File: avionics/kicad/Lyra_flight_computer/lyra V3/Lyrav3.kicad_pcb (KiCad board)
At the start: 4 copper layers, 50 x 60 mm, 110 parts, among them J1 Conn_01x10, J10 TSW-104-08-T-T-RA, J11 Screw_Terminal_01x12, J12 Screw_Terminal_01x12, J13 Conn_01x10, J2 Conn_01x02, J3 Conn_01x07, J4 Conn_01x03, J5 Conn_01x05, J6 USB_B_Micro, J8 Conn_01x05, J9 Conn_01x02, Q1 AO3401A, Q2 KY6802, Q3 KY6802, U1 AMS1117-5.0, U10 ADS1015IDGS, U11 PCF8574, U2 AMS1117-3.3, U3 W25Q64JVXGIQ, U4 BMI088, U5 MPL3115A2, U6 ADXL375BCCZ-RL7, U7 LIS3MDL, U8 RP2040, U9 ADS1015IDGS, X1 S3D12.288000B20F30T

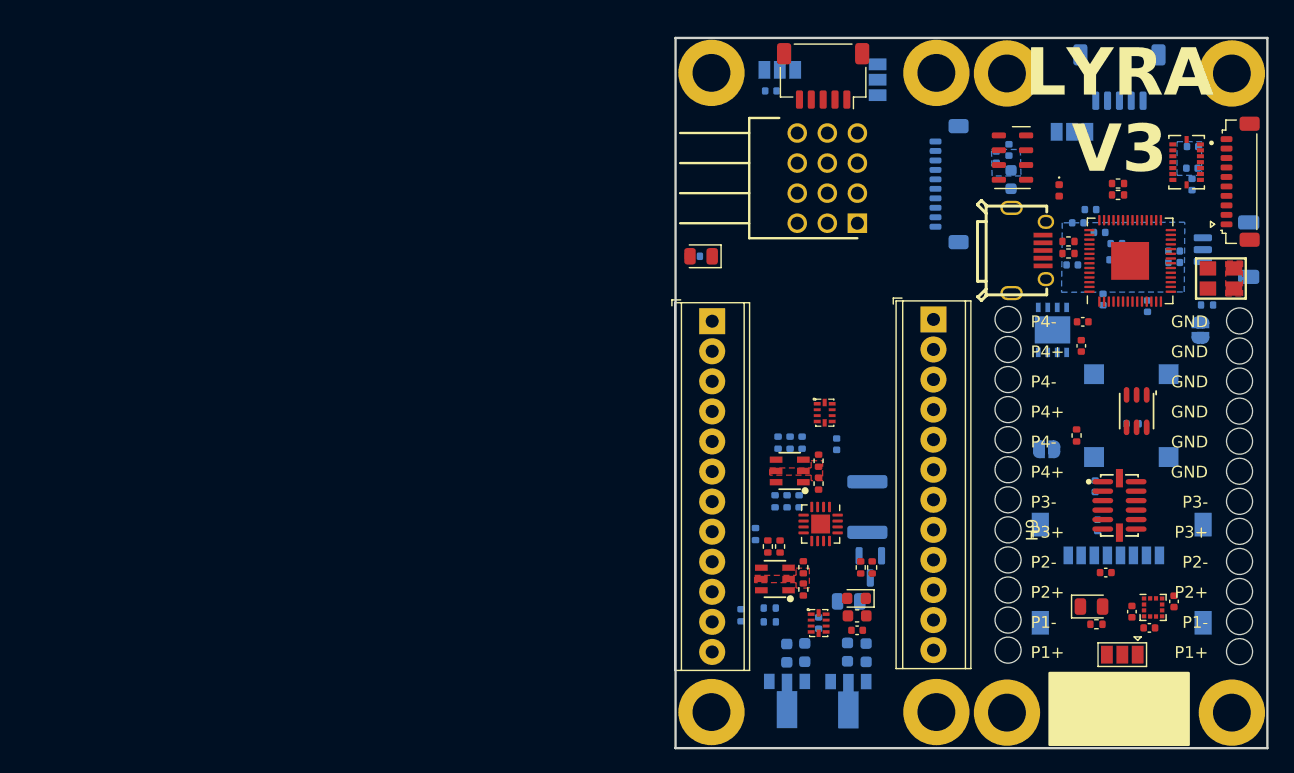
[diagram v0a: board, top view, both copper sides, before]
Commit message: simplified lyrav3
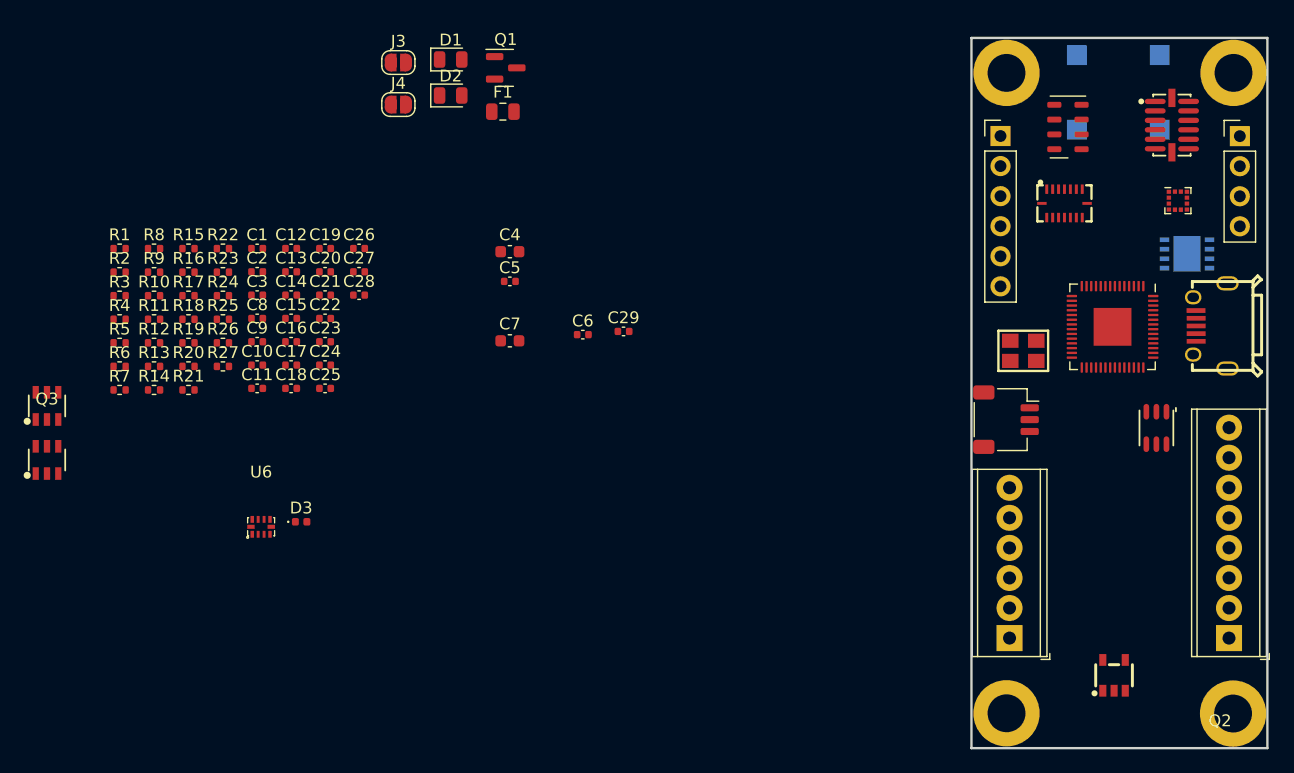
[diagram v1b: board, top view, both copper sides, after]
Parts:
- removed C30, C32: 100n, Capacitor_SMD:C_0402_1005Metric
- removed C31: 2u2, Capacitor_SMD:C_0402_1005Metric
- removed C33, C34: 1u, Capacitor_SMD:C_0402_1005Metric
- removed Card2: TF-002-H18, easyeda2kicad:SIM-SMD_TF-002-H18
- removed D4: D, Diode_SMD:D_0402_1005Metric
- removed F2: 200ma, Fuse:Fuse_0805_2012Metric
- removed FB1: FerriteBead_Small, Diode_SMD:D_0603_1608Metric
- removed H10, H9: Access Hole, customfootprints:1x10 2.54mm pitch acess hole
- removed H5, H6, H7, H8: MountingHole_Pad, MountingHole:MountingHole_3.2mm_M3_DIN965_Pad
- removed J10: TSW-104-08-T-T-RA, SamacSys_Parts:HDRRA12W64P254_3X4_1016X254X810P
- removed J11, J12: Screw_Terminal_01x12, TerminalBlock_Phoenix:TerminalBlock_Phoenix_MPT-0,5-12-2.54_1x12_P2.54mm_Horizontal
- removed J13: Conn_01x10, Connector_JST:JST_SUR_SM10B-SURS-TF_1x10-1MP_P0.80mm_Horizontal
- removed J9: Conn_01x02, Jumper:SolderJumper-2_P1.3mm_Open_RoundedPad1.0x1.5mm
- removed JP1, JP2, JP3, JP5: SolderJumper_3_Open, Jumper:SolderJumper-3_P1.3mm_Open_Pad1.0x1.5mm
- removed U1: AMS1117-5.0, Package_TO_SOT_SMD:SOT-89-3
- removed U10: ADS1015IDGS, easyeda2kicad:X2QFN-10_L2.0-W1.5-P0.50-BL
- removed U11: PCF8574, Package_DFN_QFN:WQFN-16-1EP_3x3mm_P0.5mm_EP1.6x1.6mm
- added C18: 1u, Capacitor_SMD:C_0402_1005Metric, F.Cu at (126.1, 88.6)
- added D1: LED, LED_SMD:LED_0805_2012Metric, F.Cu at (139.6, 60.8)
- added J7: USB_B_Micro, easyeda2kicad:MICRO-USB-SMD_U254-051T-4BHJ25-F2S, F.Cu at (203.8, 83.4)
- C1, C13, C15, C20, C21, C24, C25, C26, C28, C29, C9, Q1, R1: moved to F.Cu
- C10: value 10u -> 1u; footprint Capacitor_SMD:C_0603_1608Metric -> Capacitor_SMD:C_0402_1005Metric; moved to F.Cu
- C11: value 10u -> 100n; footprint Capacitor_SMD:C_0603_1608Metric -> Capacitor_SMD:C_0402_1005Metric
- C14, C22, C23: value 1u -> 100n; moved to F.Cu
- C16: value 1u -> 100n
- C19: value 100n -> 1u
- C2, C3: value 22u -> 100n; footprint Capacitor_SMD:C_0603_1608Metric -> Capacitor_SMD:C_0402_1005Metric; moved to F.Cu
- C27: value 100n -> 2u2; moved to F.Cu
- C4: value 22u -> 10u; moved to F.Cu
- C5: value 22u -> 1u; footprint Capacitor_SMD:C_0603_1608Metric -> Capacitor_SMD:C_0402_1005Metric; moved to F.Cu
- C6, C8: value 100n -> 1u; moved to F.Cu
- C7: value 100n -> 10u; footprint Capacitor_SMD:C_0402_1005Metric -> Capacitor_SMD:C_0603_1608Metric; moved to F.Cu
- D3: value LED -> D; footprint LED_SMD:LED_0805_2012Metric -> Diode_SMD:D_0402_1005Metric
- F1: value 2a -> 200ma; footprint Fuse:Fuse_1812_4532Metric -> Fuse:Fuse_0805_2012Metric; moved to F.Cu
- J1: value Conn_01x10 -> Screw_Terminal_01x08; footprint Connector_JST:JST_SUR_SM10B-SURS-TF_1x10-1MP_P0.80mm_Horizontal -> TerminalBlock_Phoenix:TerminalBlock_Phoenix_MPT-0,5-8-2.54_1x08_P2.54mm_Horizontal; moved to F.Cu
- J2: value Conn_01x02 -> Screw_Terminal_01x06; footprint Jumper:SolderJumper-2_P1.3mm_Open_RoundedPad1.0x1.5mm -> TerminalBlock_Phoenix:TerminalBlock_Phoenix_MPT-0,5-6-2.54_1x06_P2.54mm_Horizontal; moved to F.Cu
- J3: value Conn_01x07 -> Conn_01x02; footprint Connector_JST:JST_SH_SM07B-SRSS-TB_1x07-1MP_P1.00mm_Horizontal -> Jumper:SolderJumper-2_P1.3mm_Open_RoundedPad1.0x1.5mm; moved to F.Cu
- J4: value Conn_01x03 -> Conn_01x02; footprint Connector_JST:JST_SH_SM03B-SRSS-TB_1x03-1MP_P1.00mm_Horizontal -> Jumper:SolderJumper-2_P1.3mm_Open_RoundedPad1.0x1.5mm; moved to F.Cu
- J5: value Conn_01x05 -> Conn_01x03; footprint Connector_JST:JST_SH_SM05B-SRSS-TB_1x05-1MP_P1.00mm_Horizontal -> Connector_JST:JST_SH_SM03B-SRSS-TB_1x03-1MP_P1.00mm_Horizontal
- J6: value USB_B_Micro -> Conn_01x06; footprint easyeda2kicad:MICRO-USB-SMD_U254-051T-4BHJ25-F2S -> Connector_PinHeader_2.54mm:PinHeader_1x06_P2.54mm_Vertical
- J8: value Conn_01x05 -> Conn_01x04; footprint Connector_JST:JST_SH_SM05B-SRSS-TB_1x05-1MP_P1.00mm_Horizontal -> Connector_PinHeader_2.54mm:PinHeader_1x04_P2.54mm_Vertical; moved to F.Cu
- R10: value 6k -> 20k; moved to F.Cu
- R11, R23: value 470R -> 20k
- R12, R24: value 470R -> 6k
- R13: value 2k2 -> 6k
- R14: value 2k2 -> 10k
- R15: value 10R -> 27R; moved to F.Cu
- R16: value 10R -> 470R; moved to F.Cu
- R17: value 20k -> 470R
- R18: value 20k -> 27R; moved to F.Cu
- R19: value 6k -> 10R
- R2: value 20k -> 1k
- R20, R9: value 6k -> 10R; moved to F.Cu
- R21: value 27R -> 20k
- R22: value 27R -> 1k
- R25: value 10k -> 6k; moved to F.Cu
- R26, R27: value 1k -> 470R
- R3: value 6k -> 1k
- R4: value 1k -> 20k; moved to F.Cu
- R5: value 10R -> 6k; moved to F.Cu
- R6: value 10R -> 2k2; moved to F.Cu
- R7: value 20k -> 2k2; moved to F.Cu
- R8: value 20k -> 10R; moved to F.Cu
- U2: value AMS1117-3.3 -> BMI088; footprint Package_TO_SOT_SMD:SOT-89-3 -> easyeda2kicad:LGA-16_L4.5-W3.0-P0.50-BL; moved to F.Cu
- U3: value W25Q64JVXGIQ -> MPL3115A2; footprint easyeda2kicad:XSON-8_L4.0-W4.0-P0.80-TL-EP -> Package_LGA:NXP_LGA-8_3x5mm_P1.25mm_H1.1mm; moved to F.Cu
- U4: value BMI088 -> ADXL375BCCZ-RL7; footprint SnapEDA Library:PQFN50P450X300X100-16N -> easyeda2kicad:LGA-14_L5.0-W3.0-P0.80-BL
- U5: value MPL3115A2 -> LIS3MDL; footprint Package_LGA:NXP_LGA-8_3x5mm_P1.25mm_H1.1mm -> Package_LGA:LGA-12_2x2mm_P0.5mm
- U6: value ADXL375BCCZ-RL7 -> ADS1015IDGS; footprint easyeda2kicad:LGA-14_L5.0-W3.0-P0.80-BL -> easyeda2kicad:X2QFN-10_L2.0-W1.5-P0.50-BL
- U7: value LIS3MDL -> W25Q64JVXGIQ; footprint Package_LGA:LGA-12_2x2mm_P0.5mm -> easyeda2kicad:XSON-8_L4.0-W4.0-P0.80-TL-EP; moved to B.Cu
- U9: value ADS1015IDGS -> LDK130-33_SOT23_SOT353; footprint easyeda2kicad:X2QFN-10_L2.0-W1.5-P0.50-BL -> easyeda2kicad:SOT-23-5_L3.0-W1.6-P0.95-LS2.8-BL
- moved R4 86.0 mm to (111.6, 82.8)
- moved R25 83.2 mm to (120.4, 82.8), turned to 0 degrees
- moved R14 83.1 mm to (114.5, 88.8)
- moved R13 82.9 mm to (114.5, 86.8)
- moved J3 81.9 mm to (135.2, 61.1), turned to 0 degrees
- moved C8 80.0 mm to (123.3, 82.7)
- moved C17 77.2 mm to (126.1, 86.7), turned to 0 degrees
- moved R27 76.9 mm to (120.4, 86.8), turned to 0 degrees
- moved C16 76.4 mm to (126.1, 84.7), turned to 0 degrees
- moved R21 75.2 mm to (117.5, 88.8)
- moved C19 74.7 mm to (129.0, 76.8), turned to 0 degrees
- moved R26 72.5 mm to (120.4, 84.8), turned to 0 degrees
- moved U6 72.5 mm to (123.6, 100.3), turned to 0 degrees
- moved C21 71.8 mm to (129.0, 80.8)
- moved R22 71.4 mm to (120.4, 76.8), turned to 0 degrees
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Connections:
- C11 pad 1: +12VA -> +3V3
- C12 pad 1: +12VA -> +3V3
- C13 pad 1: Net-(U5-CAP) -> +3V3
- C14 pad 1: +3V3 -> Net-(U5-C1)
- C16 pad 1: +3V3 -> +1V1
- C17 pad 1: +3V3 -> +1V1
- C19 pad 1: Net-(U7-C1) -> +3V3
- C2 pad 1: +12VA -> +3V3
- C20 pad 1: +1V1 -> +3V3
- C21 pad 1: +1V1 -> +3V3
- C22 pad 1: +1V1 -> +3V3
- C29 pad 1: +3V3 -> Net-(U9-BP)
- C29 pad 2: GND -> Net-(U9-GND)
- C3 pad 1: +5VD -> +3V3
- C4 pad 1: +12VA -> +3V3
- C5 pad 1: +3V3 -> +12VA
- C5 pad 2: GND -> Net-(U9-GND)
- C6 pad 2: GND -> Net-(U9-GND)
- C7 pad 1: +3V3 -> +12VA
- C8 pad 1: +3V3 -> +12VA
- C9 pad 1: +3V3 -> Net-(U3-CAP)
- D3 pad 1: GND -> +12V
- F1 pad 1: Net-(Q1-S) -> +12P
- F1 pad 2: +12P -> +12VA
- J1 pad 1: GND -> /P4-
- J1 pad 2: /SERVO4 BOT -> /PYRO PWR
- J1 pad 3: /SERVO3 BOT -> /P3-
- J1 pad 4: /SERVO2 BOT -> /PYRO PWR
- J1 pad 5: /SERVO1 BOT -> /P2-
- J1 pad 6: /I2C1 SDA BOT -> /PYRO PWR
- J1 pad 7: /I2C1 SCL BOT -> /P1-
- J1 pad 8: +5VD -> /PYRO PWR
- J2 pad 1: /RUN -> /PYRO PWR
- J2 pad 2: GND -> +12P
- J3 pad 1: /SPI0 GPIO -> /RUN
- J3 pad 2: /SPI0 MISO -> GND
- J4 pad 1: /SWCLK -> GND
- J4 pad 2: GND -> /BOOTSEL
- J5 pad 1: /I2C GPIO -> /SWCLK
- J5 pad 2: /I2C PWR -> GND
- J5 pad 3: /I2C1 SCL BOT -> /SWD
- J6 pad 1: Net-(D4-A) -> /BRKOUT5
- J6 pad 2: /USB_D- -> /BRKOUT6
- J6 pad 3: /USB_D+ -> /BRKOUT7
- J6 pad 4: unconnected-(J6-ID-Pad4) -> +12VA
- J6 pad 5: GND -> +3V3
- J6 pad 6: unconnected-(J6-Shield-Pad6) -> GND
- J8 pad 1: /UART GPIO -> /BRKOUT4
- J8 pad 2: /UART PWR -> /BRKOUT3
- J8 pad 3: /UART0 RX -> /BRKOUT2
- J8 pad 4: /UART0 TX -> /BRKOUT1
- Q1 pad 2: Net-(Q1-S) -> +12P
- Q2 pad 1: /P1 EN BOT -> /P1 EN 
- Q2 pad 3: /P2 EN BOT -> /P2 EN 
- Q3 pad 1: /P3 EN BOT -> /P3 EN 
- Q3 pad 3: /P4 EN BOT -> /P4 EN 
- R1 pad 1: Net-(D2-A) -> Net-(D1-A)
- R10 pad 1: /P3 CONT BOT -> Net-(Q2A-D)
- R10 pad 2: GND -> /P1 CONT 
- R11 pad 1: GND -> Net-(Q3A-D)
- R11 pad 2: /P1 EN BOT -> /P3 CONT 
- R12 pad 1: GND -> /P1 CONT 
- R12 pad 2: /P3 EN BOT -> GND
- R13 pad 1: +3V3 -> /P3 CONT 
- R13 pad 2: /I2C1 SCL -> GND
- R14 pad 2: /I2C1 SDA -> /RUN
- R15 pad 1: /P2- -> /USB_D+
- R15 pad 2: Net-(Q2B-D) -> /RP USB_D+
- R16 pad 1: /P4- -> GND
- R16 pad 2: Net-(Q3B-D) -> /P1 EN 
- R17 pad 1: Net-(Q2B-D) -> GND
- R17 pad 2: /P2 CONT BOT -> /P3 EN 
- R18 pad 1: Net-(Q3B-D) -> /RP USB_D-
- R18 pad 2: /P4 CONT BOT -> /USB_D-
- R19 pad 1: /P2 CONT BOT -> /P2-
- R19 pad 2: GND -> Net-(Q2B-D)
- R2 pad 1: +12V -> Net-(LED1-+-Pad4)
- R2 pad 2: /BATT SENSE BOT -> +3V3
- R20 pad 1: /P4 CONT BOT -> /P4-
- R20 pad 2: GND -> Net-(Q3B-D)
- R21 pad 1: /USB_D+ -> Net-(Q2B-D)
- R21 pad 2: /RP USB_D+ -> /P2 CONT 
- R22 pad 1: /RP USB_D- -> /QSPI_SS
- R22 pad 2: /USB_D- -> /BOOTSEL
- R23 pad 1: GND -> Net-(Q3B-D)
- R23 pad 2: /P2 EN BOT -> /P4 CONT 
- R24 pad 1: GND -> /P2 CONT 
- R24 pad 2: /P4 EN BOT -> GND
- R25 pad 1: +3V3 -> /P4 CONT 
- R25 pad 2: /RUN -> GND
- R26 pad 1: /QSPI_SS -> GND
- R26 pad 2: /BOOTSEL -> /P2 EN 
- R27 pad 1: Net-(D3-A) -> GND
- R27 pad 2: +3V3 -> /P4 EN 
- R3 pad 1: /BATT SENSE BOT -> Net-(D2-A)
- R3 pad 2: GND -> +3V3
- R4 pad 1: Net-(LED1-+-Pad4) -> +12V
- R4 pad 2: +3V3 -> /BATT SENSE 
- R5 pad 1: /P1- -> /BATT SENSE 
- R5 pad 2: Net-(Q2A-D) -> GND
- R6 pad 1: /P3- -> +3V3
- R6 pad 2: Net-(Q3A-D) -> /I2C1 SCL
- R7 pad 1: Net-(Q2A-D) -> +3V3
- R7 pad 2: /P1 CONT BOT -> /I2C1 SDA
- R8 pad 1: Net-(Q3A-D) -> /P1-
- R8 pad 2: /P3 CONT BOT -> Net-(Q2A-D)
- R9 pad 1: /P1 CONT BOT -> /P3-
- R9 pad 2: GND -> Net-(Q3A-D)
- U2 pad 1: GND -> unconnected-(U2-INT2-Pad1)
- U2 pad 2: +3V3 -> unconnected-(U2-NC-Pad2)
- U2 pad 3: +12VA -> +3V3
- U3 pad 1: /QSPI_SS -> +3V3
- U3 pad 2: /QSPI_SD1 -> Net-(U3-CAP)
- U3 pad 3: /QSPI_SD2 -> GND
- U3 pad 4: GND -> +3V3
- U3 pad 5: /QSPI_SDO -> unconnected-(U3-INT2-Pad5)
- U3 pad 6: /QSPI_SCLK -> unconnected-(U3-INT1-Pad6)
- U3 pad 7: /QSPI_SD3 -> /I2C0 SDA
- U3 pad 8: +3V3 -> /I2C0 SCL
- U4 pad 1: unconnected-(U4-INT2-Pad1) -> +3V3
- U4 pad 10: GND -> unconnected-(U4-NC-Pad10)
- U4 pad 11: +3V3 -> GND
- U4 pad 12: unconnected-(U4-INT3-Pad12) -> GND
- U4 pad 13: unconnected-(U4-INT4-Pad13) -> /I2C0 SDA
- U4 pad 14: +3V3 -> /I2C0 SCL
- U4 pad 2: unconnected-(U4-NC-Pad2) -> GND
- U4 pad 5: unconnected-(U4-CSB2-Pad5) -> GND
- U4 pad 6: GND -> +3V3
- U4 pad 8: /I2C0 SCL -> unconnected-(U4-INT1-Pad8)
- U4 pad 9: /I2C0 SDA -> unconnected-(U4-INT2-Pad9)
- U5 pad 1: +3V3 -> /I2C0 SCL
- U5 pad 2: Net-(U5-CAP) -> GND
- U5 pad 4: +3V3 -> Net-(U5-C1)
- U5 pad 5: unconnected-(U5-INT2-Pad5) -> +3V3
- U5 pad 6: unconnected-(U5-INT1-Pad6) -> +3V3
- U5 pad 7: /I2C0 SDA -> unconnected-(U5-INT-Pad7)
- U5 pad 8: /I2C0 SCL -> unconnected-(U5-DRDY-Pad8)
- U6 pad 10: unconnected-(U6-NC-Pad10) -> /I2C1 SCL
- U6 pad 2: GND -> unconnected-(U6-ALERT/RDY-Pad2)
- U6 pad 3: +3V3 -> GND
- U6 pad 4: GND -> /P1 CONT 
- U6 pad 5: GND -> /P2 CONT 
- U6 pad 6: +3V3 -> /P3 CONT 
- U6 pad 7: +3V3 -> /P4 CONT 
- U6 pad 8: unconnected-(U6-INT1-Pad8) -> +3V3
- U6 pad 9: unconnected-(U6-INT2-Pad9) -> /I2C1 SDA
- U7 pad 1: /I2C0 SCL -> /QSPI_SS
- U7 pad 2: GND -> /QSPI_SD1
- U7 pad 3: GND -> /QSPI_SD2
- U7 pad 4: Net-(U7-C1) -> GND
- U7 pad 5: +3V3 -> /QSPI_SDO
- U7 pad 6: +3V3 -> /QSPI_SCLK
- U7 pad 7: unconnected-(U7-INT-Pad7) -> /QSPI_SD3
- U7 pad 8: unconnected-(U7-DRDY-Pad8) -> +3V3
- U7 pad 9: GND -> unconnected-(U7-EP-Pad9)
- U8 pad 12: /LEDRED -> unconnected-(U8-GPIO9-Pad12)
- U8 pad 13: /LEDGREEN -> unconnected-(U8-GPIO10-Pad13)
- U8 pad 14: /LEDBLUE -> unconnected-(U8-GPIO11-Pad14)
- U8 pad 15: /SERVO1 -> unconnected-(U8-GPIO12-Pad15)
- U8 pad 16: /SERVO2 -> /BRKOUT5
- U8 pad 17: /SERVO3 -> /BRKOUT6
- U8 pad 18: /SERVO4 -> /BRKOUT7
- U8 pad 2: /SPI0 GPIO -> /BRKOUT1
- U8 pad 27: /UART0 TX -> unconnected-(U8-GPIO16-Pad27)
- U8 pad 28: /UART0 RX -> unconnected-(U8-GPIO17-Pad28)
- U8 pad 29: /SPI0 SCK -> unconnected-(U8-GPIO18-Pad29)
- U8 pad 3: unconnected-(U8-GPIO1-Pad3) -> /BRKOUT2
- U8 pad 30: /SPI0 MISO -> unconnected-(U8-GPIO19-Pad30)
- U8 pad 31: /SPI0 MOSI -> unconnected-(U8-GPIO20-Pad31)
- U8 pad 32: /SPI0 CSn -> unconnected-(U8-GPIO21-Pad32)
- U8 pad 34: /I2C1 SDA -> unconnected-(U8-GPIO22-Pad34)
- U8 pad 35: /I2C1 SCL -> /LEDRED
- U8 pad 36: /UART GPIO -> /LEDGREEN
- U8 pad 37: unconnected-(U8-GPIO25-Pad37) -> /LEDBLUE
- U8 pad 4: /SD CS -> /BRKOUT3
- U8 pad 40: unconnected-(U8-GPIO28_ADC2-Pad40) -> /BATT SENSE 
- U8 pad 5: unconnected-(U8-GPIO3-Pad5) -> /BRKOUT4
- U9 pad 1: +3V3 -> +12VA
- U9 pad 2: unconnected-(U9-ALERT/RDY-Pad2) -> Net-(U9-GND)
- U9 pad 3: GND -> +12VA
- U9 pad 4: /P3 CONT BOT -> Net-(U9-BP)
- U9 pad 5: /P4 CONT BOT -> +3V3
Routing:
- removed copper zone on B.Cu, net +3V3
- removed copper zone on F.Cu, net +3V3
- removed copper zone on B.Cu, net GND
- removed copper zone on F.Cu, net GND
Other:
- board size 50 x 60 mm -> 25 x 60 mm
- board text removed: "GND"
- board text removed: "LYRA V3"
- board text removed: "P1+"
- board text removed: "P1-"
- board text removed: "P2+"
- board text removed: "P2-"
- board text removed: "P3+"
- board text removed: "P3-"
- board text removed: "P4+"
- board text removed: "P4-"
- board text removed: "PRS"
